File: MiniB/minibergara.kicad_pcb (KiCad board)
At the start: 2 copper layers, 13 parts, among them SW1 SW_Nidec_CAS-120A1, U1 TB6612_BREAKOUT, U2 LM7805_TO220

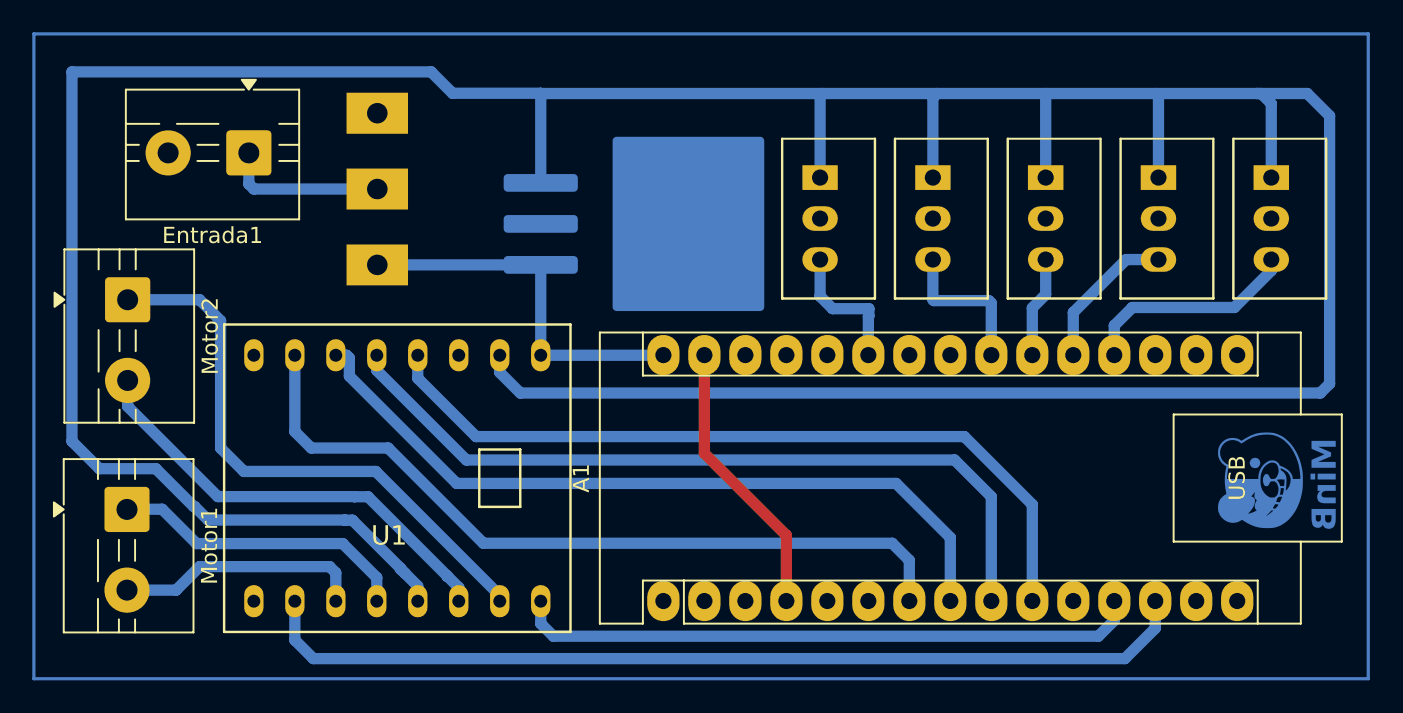
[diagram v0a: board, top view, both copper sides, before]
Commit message: boton y led puestos
hola
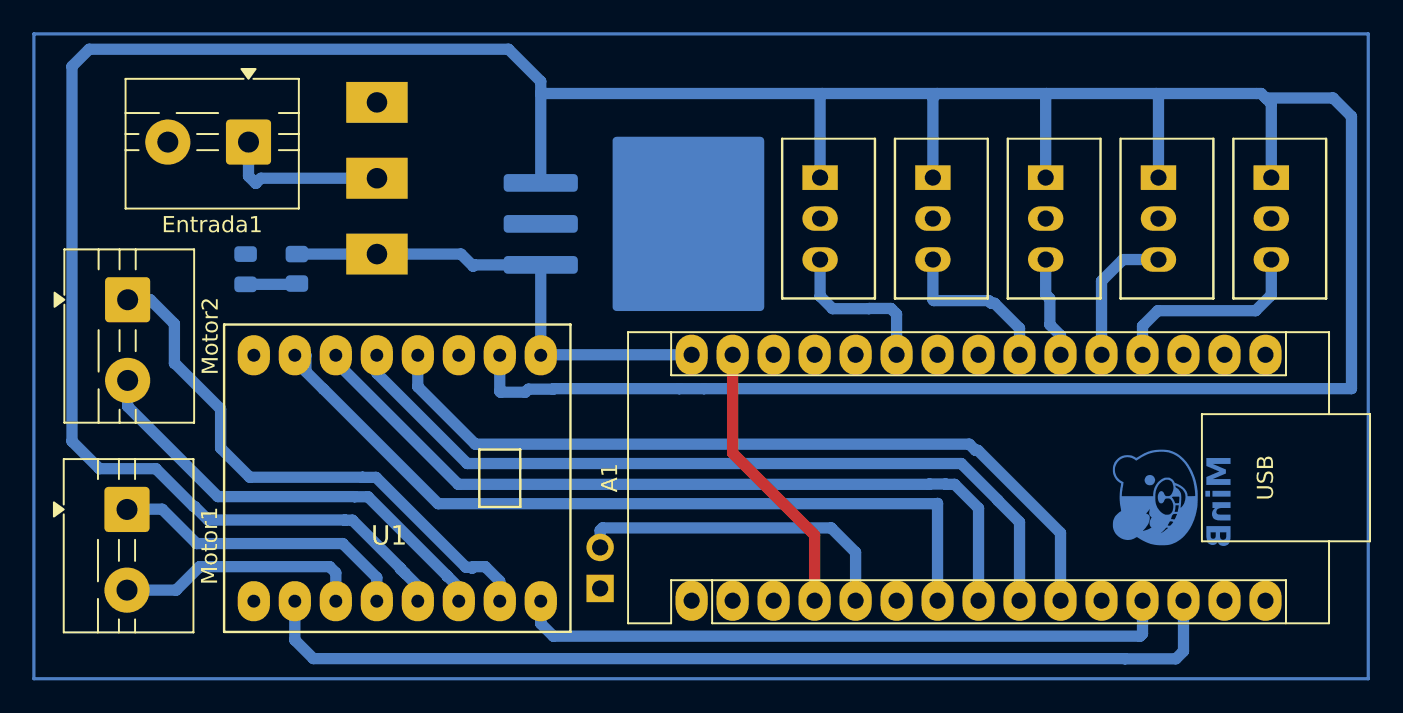
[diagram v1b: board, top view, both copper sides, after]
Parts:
- added D1: LED, LED_SMD:LED_0805_2012Metric, B.Cu at (86.0, 71.2)
- added J1: boton, Connector_PinHeader_2.54mm:PinHeader_1x02_P2.54mm_Vertical, B.Cu at (108.0, 91.0)
- added R1: R, Resistor_SMD:R_0805_2012Metric, B.Cu at (89.2, 71.2)
- moved G*** 6.60 mm to (142.2, 85.4)
- moved A1 1.75 mm to (113.7, 91.7)
- moved Entrada1 0.67 mm to (86.2, 63.3)
- moved SW1 0.67 mm to (94.2, 65.5)
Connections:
- A1 pad 5: unconnected-(A1-D2-Pad5) -> d2
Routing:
- net d2: track 0.00 -> 20.6 mm
- net VCC: track 23.3 -> 30.4 mm
- net +5V: track 230.7 -> 235.3 mm
- net Net-(D1-A): track 0.00 -> 3.20 mm
- net PWMB: track 58.7 -> 61.3 mm
- net B1: track 47.3 -> 49.7 mm
- net PWMA: track 38.9 -> 41.1 mm
- net B2: track 48.6 -> 50.3 mm
- net Sh1: track 8.51 -> 10.0 mm
- net M2a: track 35.6 -> 34.5 mm
- net A1: track 48.7 -> 49.7 mm
- net A2: track 48.7 -> 49.6 mm
- net out1: track 13.7 -> 12.8 mm
- net Sh2: track 9.41 -> 10.2 mm
- net out2: track 9.28 -> 8.65 mm
